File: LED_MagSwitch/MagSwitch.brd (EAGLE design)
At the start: 29.5 x 28 mm, 6 parts, among them X1 MSTBA2, X2 MSTBA4

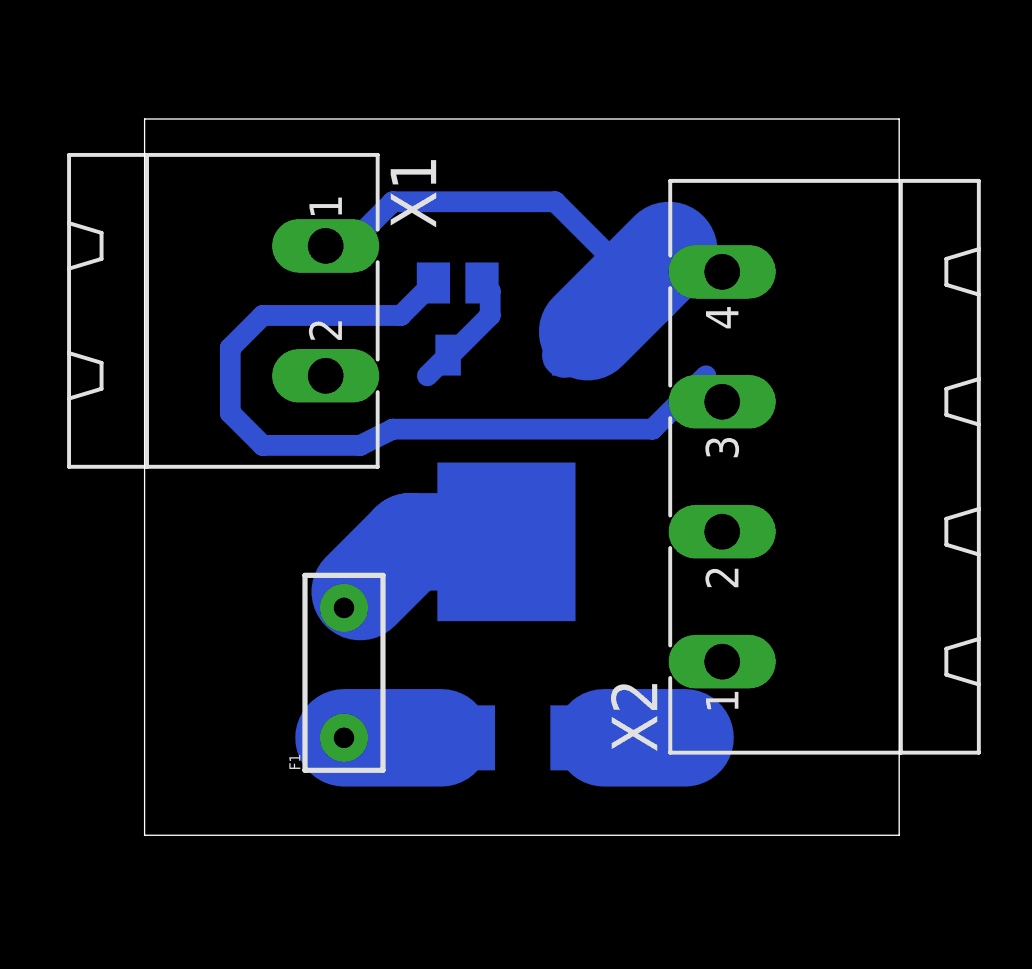
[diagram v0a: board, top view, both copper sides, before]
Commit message: MagSwitch ready to prototype!
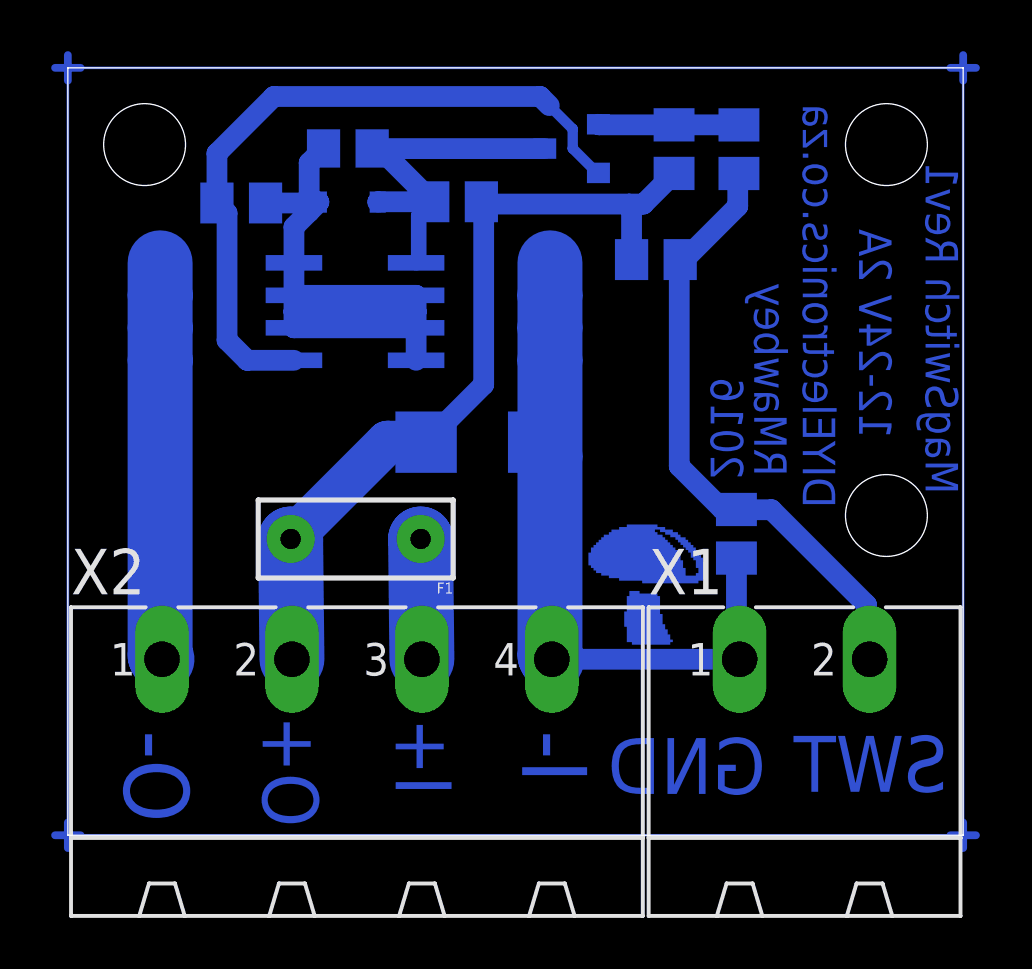
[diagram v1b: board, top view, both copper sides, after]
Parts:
- added C1: 100nF, resistor:C0805
- added Q1: MMBT2222A, SparkFun-DiscreteSemi:SOT23-3
- added R2, R3: 10k, resistor:M0805
- added R4, R5, R6: 1k, resistor:M0805
- added U$2: DMG4466SSS, RobThePyro:SO08
- added U$3: DIODE_TVS_BISM6T30CAY, RobThePyro:SMB-DIODE
- added U$4: SHROOM5MM, RobThePyro:SHROOM
- D1: value (none) -> DIODE-ZENER15V; device adafruit:SMADIODE -> RobThePyro:SOD-323
- R1: value 10k -> 5k6
- U$1: value NTD5806N -> DMG4466SSS; device RobThePyro:TO252 -> RobThePyro:SO08
- moved X1 30.3 mm to (28.8, 1.80), turned to 0 degrees
- moved X2 23.1 mm to (11.3, 1.80), turned to 0 degrees
- moved D1 22.0 mm to (11.0, 24.8), turned to 0 degrees
- moved U$1 12.7 mm to (6.22, 20.5), turned to 270 degrees
- moved F1 5.25 mm to (11.3, 11.6), turned to 180 degrees
- moved R1 3.18 mm to (15.2, 24.8), turned to 0 degrees
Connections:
- new net N$4: Q1.2, R2.1, U$1.4
- new net N$6: F1.P$1, X2.3
- new net N$7: C1.1, D1.C, Q1.3, R1.2, U$2.4
- net +24V: now also F1.P$2, R3.1, R5.2, U$3.C; no longer X2.3
- net GND: now also R6.1, U$2.5, U$2.6, U$2.7, U$2.8, U$3.A; no longer U$1.2
- net N$1: now also R4.2, R5.1, R6.2, X1.2; no longer D1.A, X2.1
- net N$2: now also Q1.1, R3.2, R4.1; no longer R1.2, U$1.1, X1.2
- net N$3: now also C1.2, D1.A, R2.2, U$1.1, U$1.2, U$1.3, U$2.1, U$2.2, U$2.3; no longer D1.C, F1.P$1
- net OUT-: now also U$1.5, U$1.6, U$1.7, U$1.8, X2.1; no longer F1.P$2, U$1.3
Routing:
- net N$5: track 0.00 -> 132.0 mm
- net N$4: track 0.00 -> 27.9 mm
- net N$3: track 4.64 -> 27.2 mm
- net N$1: track 4.00 -> 24.2 mm
- net N$7: track 0.00 -> 14.8 mm
- net OUT-: track 7.42 -> 15.5 mm
- net GND: track 20.0 -> 27.6 mm
- net N$6: track 0.00 -> 4.70 mm
- net N$9: track 0.00 -> 1.00 mm
- net N$8: track 0.00 -> 1.00 mm
- net N$14: track 0.00 -> 1.00 mm
- net N$12: track 0.00 -> 1.00 mm
- net N$11: track 0.00 -> 1.00 mm
- net N$10: track 0.00 -> 1.00 mm
- net N$2: track 4.84 -> 5.50 mm
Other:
- board size 29.5 x 28 mm -> 35 x 30 mm
- board text added: "12-24V 2A"
- board text added: "2016"
- board text added: "DIYElectronics.co.za"
- board text added: "GND"
- board text added: "I+"
- board text added: "I-"
- board text added: "MagSwitch Rev1"
- board text added: "O+"
- board text added: "O-"
- board text added: "RMawbey"
- board text added: "SWT"
